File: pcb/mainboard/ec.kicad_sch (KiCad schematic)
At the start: 28 parts, among them J301 Conn_01x06_MountingPin, U301 LPC5500_FBD64, U302 74LS154, Y301 16MHz

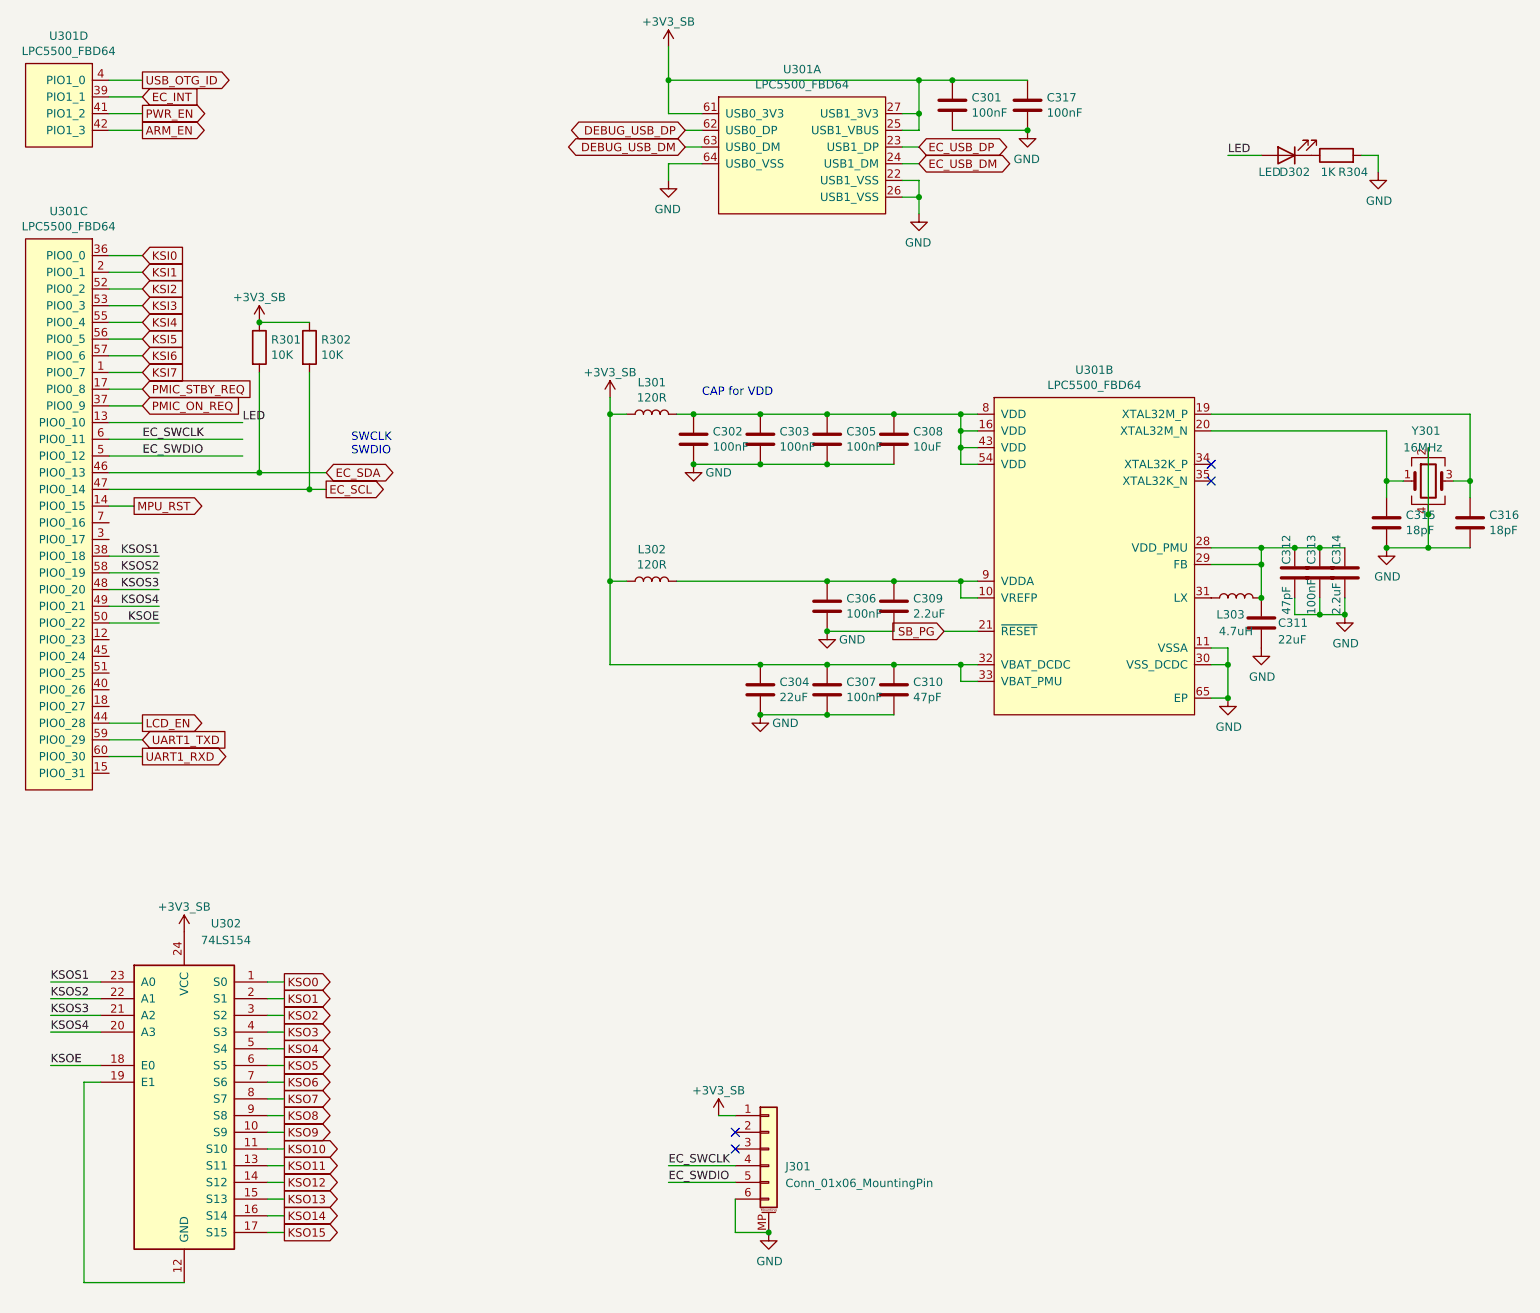
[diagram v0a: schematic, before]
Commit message: - pcb: finishing layout r0p1
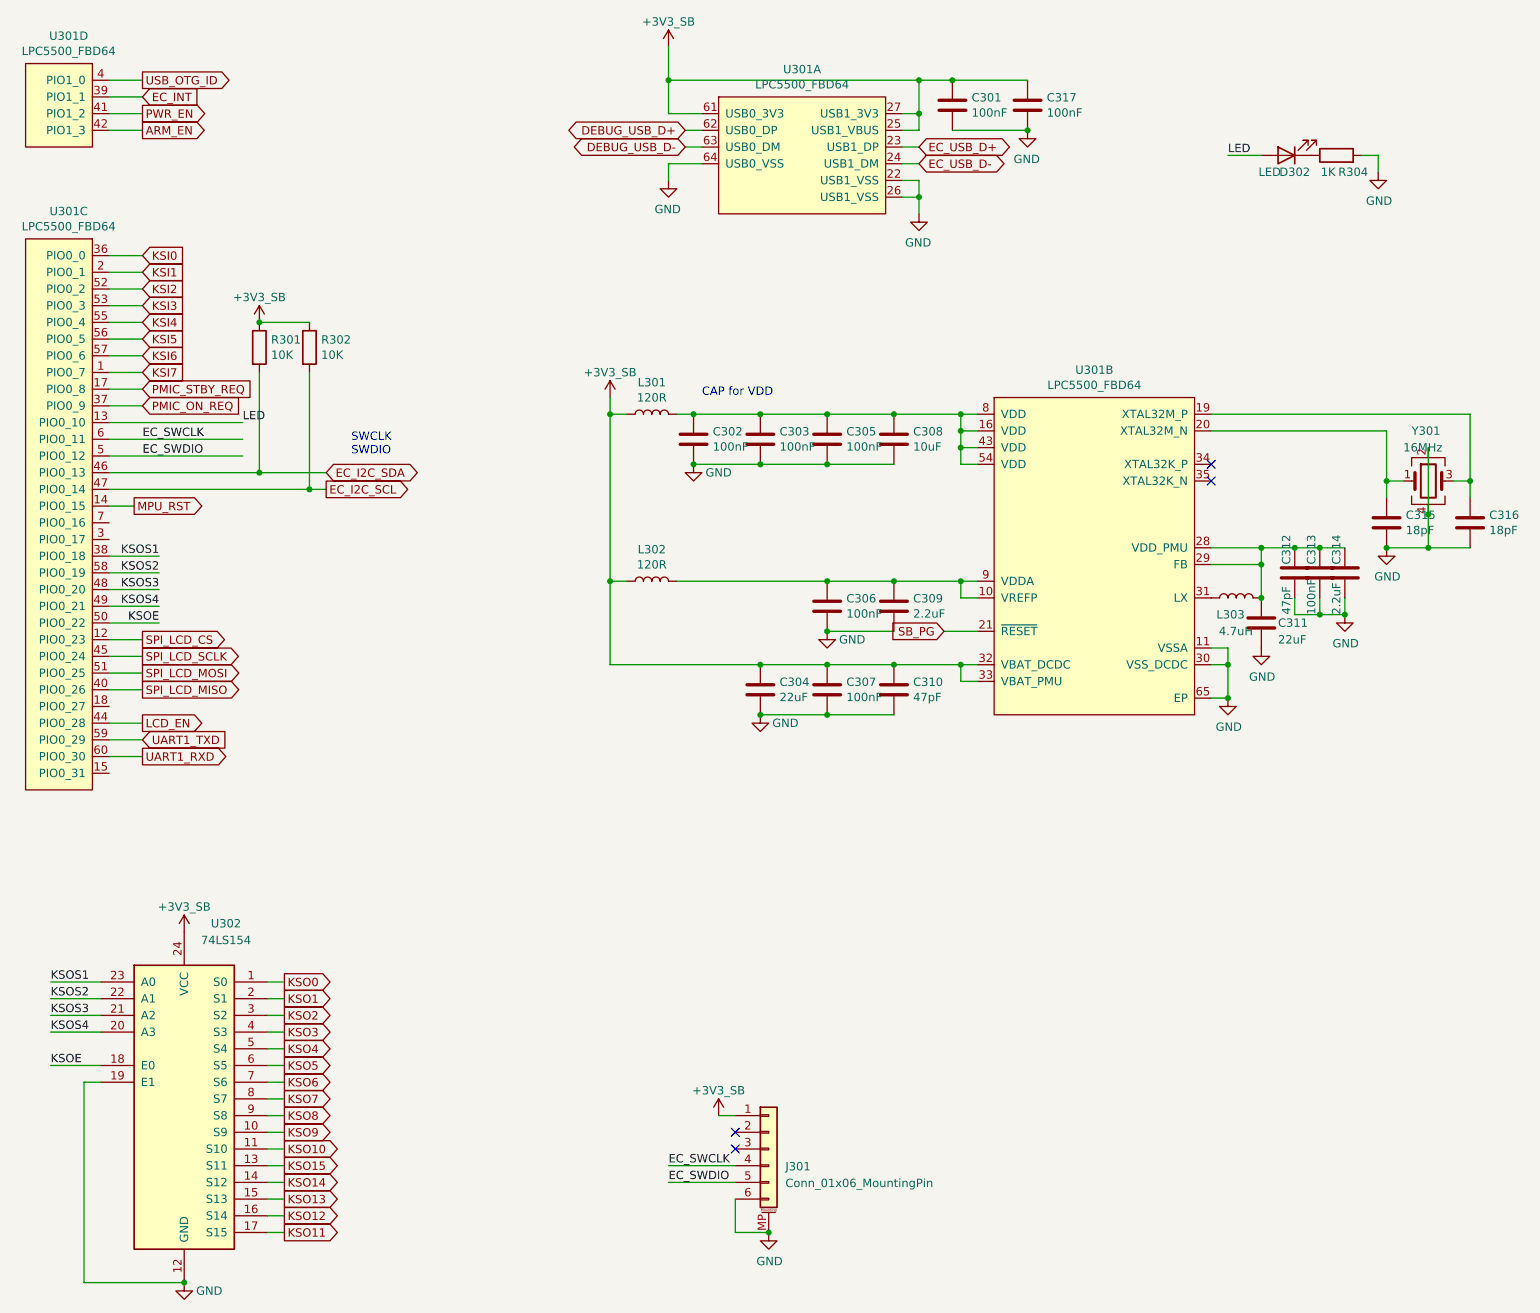
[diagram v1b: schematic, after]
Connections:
- net GND: now also U302.12 (GND), U302.19 (E1)
- net KSO11: now also U302.17 (S15); no longer U302.13 (S11)
- net KSO12: now also U302.16 (S14); no longer U302.14 (S12)
- net KSO14: now also U302.14 (S12); no longer U302.16 (S14)
- net KSO15: now also U302.13 (S11); no longer U302.17 (S15)
- net SPI_LCD_CS: now reaches U301.12 (PIO0_23)
- net SPI_LCD_MISO: now reaches U301.40 (PIO0_26)
- net SPI_LCD_SCLK: now reaches U301.45 (PIO0_24)
- net SPI_LCD_MOSI: now reaches U301.51 (PIO0_25)
- net DEBUG_USB_DM renamed DEBUG_USB_D-
- net DEBUG_USB_DP renamed DEBUG_USB_D+
- net EC_SCL renamed EC_I2C_SCL
- net EC_SDA renamed EC_I2C_SDA
- net EC_USB_DM renamed EC_USB_D-
- net EC_USB_DP renamed EC_USB_D+
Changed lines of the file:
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@@
     (comment 4 "This source describes Open Hardware and is licensed under the CERN-OHL-S v2.")
   )
+  (junction (at 64.77 224.79) (diameter 0.9144) (color 0 0 0 0))
   (junction (at 76.2 78.74) (diameter 0.9144) (color 0 0 0 0))
   (junction (at 76.2 101.6) (diameter 0.9144) (color 0 0 0 0))
@@
     (stroke (width 0) (type solid) (color 0 0 0 0))
   )
+  (wire (pts (xy 53.34 127) (xy 58.42 127))
+    (stroke (width 0) (type solid) (color 0 0 0 0))
+  )
+  (wire (pts (xy 53.34 129.54) (xy 58.42 129.54))
+    (stroke (width 0) (type solid) (color 0 0 0 0))
+  )
+  (wire (pts (xy 53.34 132.08) (xy 58.42 132.08))
+    (stroke (width 0) (type solid) (color 0 0 0 0))
+  )
+  (wire (pts (xy 53.34 134.62) (xy 58.42 134.62))
+    (stroke (width 0) (type solid) (color 0 0 0 0))
+  )
   (wire (pts (xy 53.34 139.7) (xy 58.42 139.7))
     (stroke (width 0) (type solid) (color 0 0 0 0))
@@
     )
   )
+  (global_label "SPI_LCD_CS" (shape output) (at 58.42 127 0) (fields_autoplaced)
+    (effects (font (size 1.27 1.27)) (justify left))
+    (property "Intersheet References" "${INTERSHEET_REFS}" (id 0) (at 71.9002 126.9206 0)
+      (effects (font (size 1.27 1.27)) (justify left) hide)
+    )
+  )
+  (global_label "SPI_LCD_SCLK" (shape output) (at 58.42 129.54 0) (fields_autoplaced)
+    (effects (font (size 1.27 1.27)) (justify left))
+    (property "Intersheet References" "${INTERSHEET_REFS}" (id 0) (at 74.1983 129.4606 0)
+      (effects (font (size 1.27 1.27)) (justify left) hide)
+    )
+  )
+  (global_label "SPI_LCD_MOSI" (shape output) (at 58.42 132.08 0) (fields_autoplaced)
+    (effects (font (size 1.27 1.27)) (justify left))
+    (property "Intersheet References" "${INTERSHEET_REFS}" (id 0) (at 74.0169 132.0006 0)
+      (effects (font (size 1.27 1.27)) (justify left) hide)
+    )
+  )
+  (global_label "SPI_LCD_MISO" (shape output) (at 58.42 134.62 0) (fields_autoplaced)
+    (effects (font (size 1.27 1.27)) (justify left))
+    (property "Intersheet References" "${INTERSHEET_REFS}" (id 0) (at 74.0169 134.5406 0)
+      (effects (font (size 1.27 1.27)) (justify left) hide)
+    )
+  )
   (global_label "LCD_EN" (shape output) (at 58.42 139.7 0) (fields_autoplaced)
     (effects (font (size 1.27 1.27)) (justify left))
@@
     )
   )
-  (global_label "KSO11" (shape output) (at 80.01 207.01 0) (fields_autoplaced)
-    (effects (font (size 1.27 1.27)) (justify left))
-    (property "Intersheet References" "${INTERSHEET_REFS}" (id 0) (at 87.4426 206.9306 0)
-      (effects (font (size 1.27 1.27)) (justify left) hide)
-    )
-  )
-  (global_label "KSO12" (shape output) (at 80.01 209.55 0) (fields_autoplaced)
-    (effects (font (size 1.27 1.27)) (justify left))
-    (property "Intersheet References" "${INTERSHEET_REFS}" (id 0) (at 87.4426 209.4706 0)
+  (global_label "KSO15" (shape output) (at 80.01 207.01 0) (fields_autoplaced)
+    (effects (font (size 1.27 1.27)) (justify left))
+    (property "Intersheet References" "${INTERSHEET_REFS}" (id 0) (at 87.4426 207.0894 0)
+      (effects (font (size 1.27 1.27)) (justify left) hide)
+    )
+  )
+  (global_label "KSO14" (shape output) (at 80.01 209.55 0) (fields_autoplaced)
+    (effects (font (size 1.27 1.27)) (justify left))
+    (property "Intersheet References" "${INTERSHEET_REFS}" (id 0) (at 87.4426 209.6294 0)
       (effects (font (size 1.27 1.27)) (justify left) hide)
     )
@@
   (global_label "KSO13" (shape output) (at 80.01 212.09 0) (fields_autoplaced)
     (effects (font (size 1.27 1.27)) (justify left))
-    (property "Intersheet References" "${INTERSHEET_REFS}" (id 0) (at 87.4426 212.0106 0)
-      (effects (font (size 1.27 1.27)) (justify left) hide)
-    )
-  )
-  (global_label "KSO14" (shape output) (at 80.01 214.63 0) (fields_autoplaced)
-    (effects (font (size 1.27 1.27)) (justify left))
-    (property "Intersheet References" "${INTERSHEET_REFS}" (id 0) (at 87.4426 214.5506 0)
-      (effects (font (size 1.27 1.27)) (justify left) hide)
-    )
-  )
-  (global_label "KSO15" (shape output) (at 80.01 217.17 0) (fields_autoplaced)
-    (effects (font (size 1.27 1.27)) (justify left))
-    (property "Intersheet References" "${INTERSHEET_REFS}" (id 0) (at 87.4426 217.0906 0)
-      (effects (font (size 1.27 1.27)) (justify left) hide)
-    )
-  )
-  (global_label "EC_SDA" (shape bidirectional) (at 86.36 101.6 0) (fields_autoplaced)
-    (effects (font (size 1.27 1.27)) (justify left))
-    (property "Intersheet References" "${INTERSHEET_REFS}" (id 0) (at 95.7279 101.5206 0)
-      (effects (font (size 1.27 1.27)) (justify left) hide)
-    )
-  )
-  (global_label "EC_SCL" (shape output) (at 86.36 104.14 0) (fields_autoplaced)
-    (effects (font (size 1.27 1.27)) (justify left))
-    (property "Intersheet References" "${INTERSHEET_REFS}" (id 0) (at 95.6674 104.0606 0)
-      (effects (font (size 1.27 1.27)) (justify left) hide)
-    )
-  )
-  (global_label "DEBUG_USB_DP" (shape bidirectional) (at 140.97 49.53 180)
+    (property "Intersheet References" "${INTERSHEET_REFS}" (id 0) (at 87.4426 212.1694 0)
+      (effects (font (size 1.27 1.27)) (justify left) hide)
+    )
+  )
+  (global_label "KSO12" (shape output) (at 80.01 214.63 0) (fields_autoplaced)
+    (effects (font (size 1.27 1.27)) (justify left))
+    (property "Intersheet References" "${INTERSHEET_REFS}" (id 0) (at 87.4426 214.7094 0)
+      (effects (font (size 1.27 1.27)) (justify left) hide)
+    )
+  )
+  (global_label "KSO11" (shape output) (at 80.01 217.17 0) (fields_autoplaced)
+    (effects (font (size 1.27 1.27)) (justify left))
+    (property "Intersheet References" "${INTERSHEET_REFS}" (id 0) (at 87.4426 217.2494 0)
+      (effects (font (size 1.27 1.27)) (justify left) hide)
+    )
+  )
+  (global_label "EC_I2C_SDA" (shape bidirectional) (at 86.36 101.6 0) (fields_autoplaced)
+    (effects (font (size 1.27 1.27)) (justify left))
+    (property "Intersheet References" "${INTERSHEET_REFS}" (id 0) (at 99.7798 101.5206 0)
+      (effects (font (size 1.27 1.27)) (justify left) hide)
+    )
+  )
+  (global_label "EC_I2C_SCL" (shape output) (at 86.36 104.14 0) (fields_autoplaced)
+    (effects (font (size 1.27 1.27)) (justify left))
+    (property "Intersheet References" "${INTERSHEET_REFS}" (id 0) (at 99.7193 104.0606 0)
+      (effects (font (size 1.27 1.27)) (justify left) hide)
+    )
+  )
+  (global_label "DEBUG_USB_D+" (shape bidirectional) (at 140.97 49.53 180)
     (effects (font (size 1.27 1.27)) (justify right))
     (property "Intersheet References" "${INTERSHEET_REFS}" (id 0) (at 351.79 148.59 0)
@@
     )
   )
-  (global_label "DEBUG_USB_DM" (shape bidirectional) (at 140.97 52.07 180)
+  (global_label "DEBUG_USB_D-" (shape bidirectional) (at 140.97 52.07 180)
     (effects (font (size 1.27 1.27)) (justify right))
     (property "Intersheet References" "${INTERSHEET_REFS}" (id 0) (at 351.79 148.59 0)
@@
     )
   )
-  (global_label "EC_USB_DP" (shape bidirectional) (at 176.53 52.07 0)
+  (global_label "EC_USB_D+" (shape bidirectional) (at 176.53 52.07 0)
     (effects (font (size 1.27 1.27)) (justify left))
     (property "Intersheet References" "${INTERSHEET_REFS}" (id 0) (at -34.29 151.13 0)
@@
     )
   )
-  (global_label "EC_USB_DM" (shape bidirectional) (at 176.53 54.61 0)
+  (global_label "EC_USB_D-" (shape bidirectional) (at 176.53 54.61 0)
     (effects (font (size 1.27 1.27)) (justify left))
     (property "Intersheet References" "${INTERSHEET_REFS}" (id 0) (at -34.29 151.13 0)
@@
   (symbol (lib_id "symbols:+3V3_SB") (at 64.77 171.45 0) (unit 1)
     (in_bom yes) (on_board yes) (fields_autoplaced)
-    (property "Reference" "#PWR071" (id 0) (at 64.77 175.26 0)
+    (property "Reference" "#PWR0166" (id 0) (at 64.77 175.26 0)
       (effects (font (size 1.27 1.27)) hide)
     )
@@
       (effects (font (size 1.27 1.27)) hide)
     )
+    (pin "1")
+  )
+  (symbol (lib_id "power:GND") (at 64.77 224.79 0) (unit 1)
+    (in_bom yes) (on_board yes)
+    (property "Reference" "#PWR0163" (id 0) (at 64.77 231.14 0)
+      (effects (font (size 1.27 1.27)) hide)
+    )
+    (property "Value" "GND" (id 1) (at 68.58 226.06 0))
+    (property "Footprint" "" (id 2) (at 64.77 224.79 0)
+      (effects (font (size 1.27 1.27)) hide)
+    )
+    (property "Datasheet" "" (id 3) (at 64.77 224.79 0)
+      (effects (font (size 1.27 1.27)) hide)
+    )
